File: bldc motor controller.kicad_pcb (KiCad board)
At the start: 4 copper layers, 26 x 26 mm, 55 parts, among them J1 Conn_01x04_Pin, M2 MountingHole_2.2mm_M2_DIN965_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, U1 C47023655, U2 ISM330DHCXTR, U3 C529358, U6 LIS2MDLTR

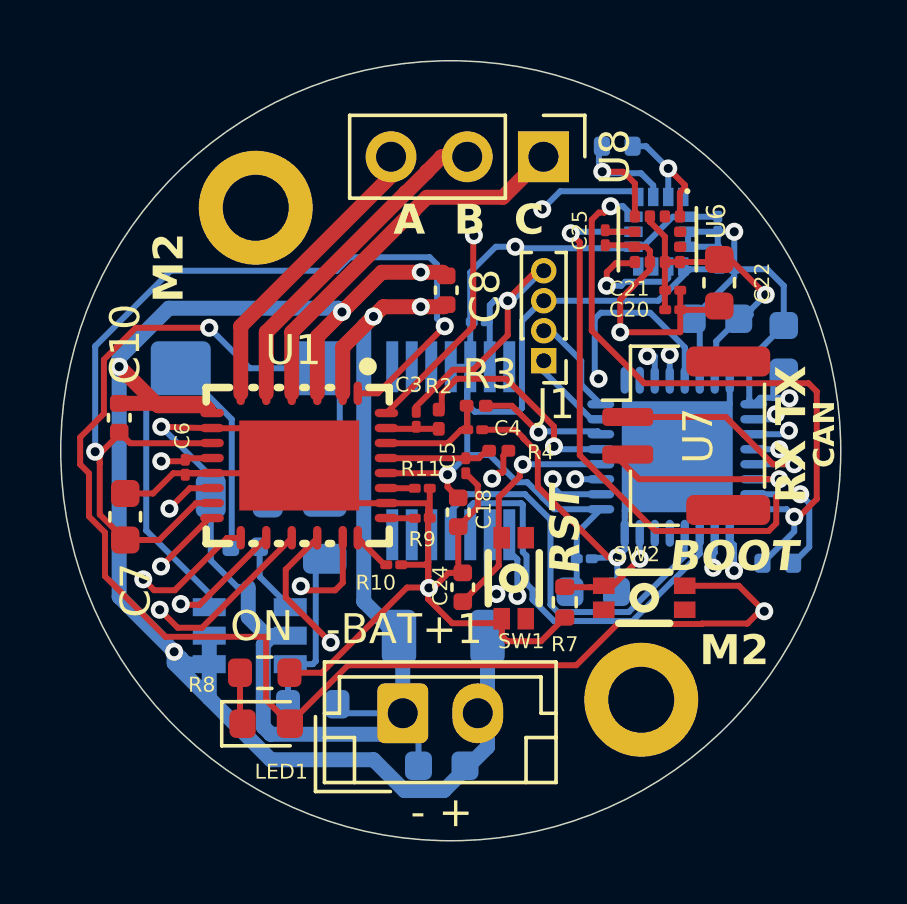
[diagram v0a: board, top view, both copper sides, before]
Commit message: Final push of the day
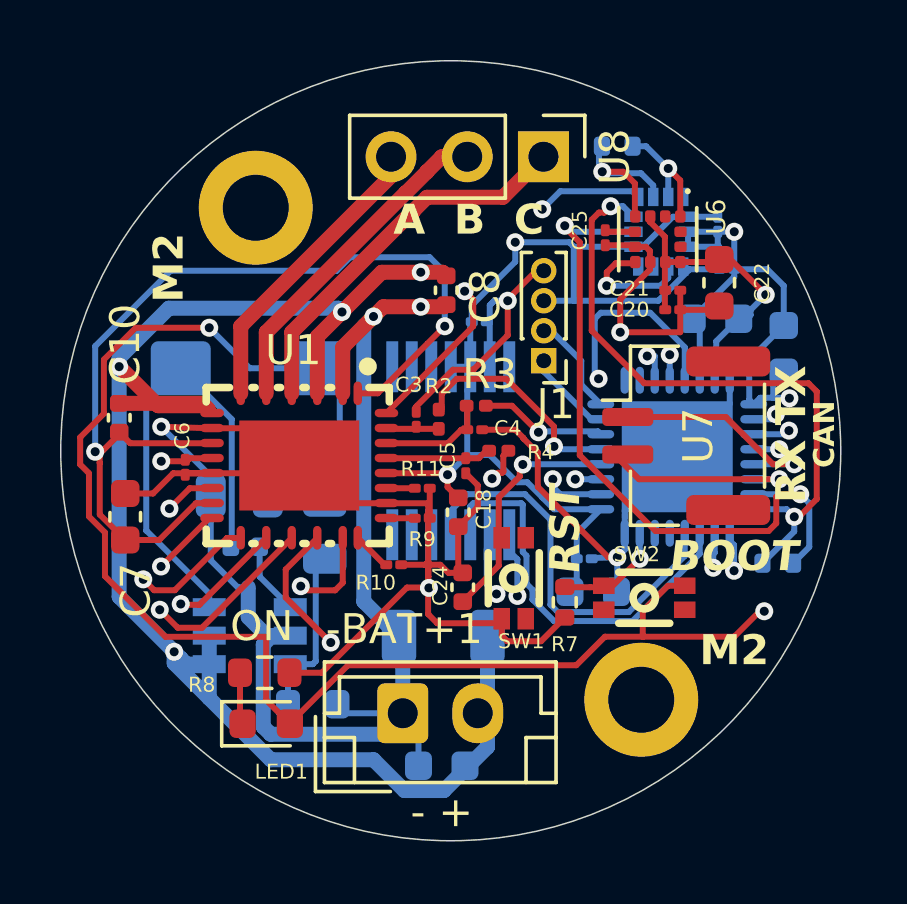
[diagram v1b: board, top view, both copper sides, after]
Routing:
- net +3.3V: track 152.4 -> 134.0 mm
- net I-LIMIT: track 24.1 -> 20.6 mm
- net GND: track 93.2 -> 92.1 mm
- net SCL1: track 23.3 -> 23.9 mm
